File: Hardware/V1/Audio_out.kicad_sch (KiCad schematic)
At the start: 30 parts, among them J0 0, J1 SJ2-3514A-SMT-TR, Q1 BC817-25-QVL

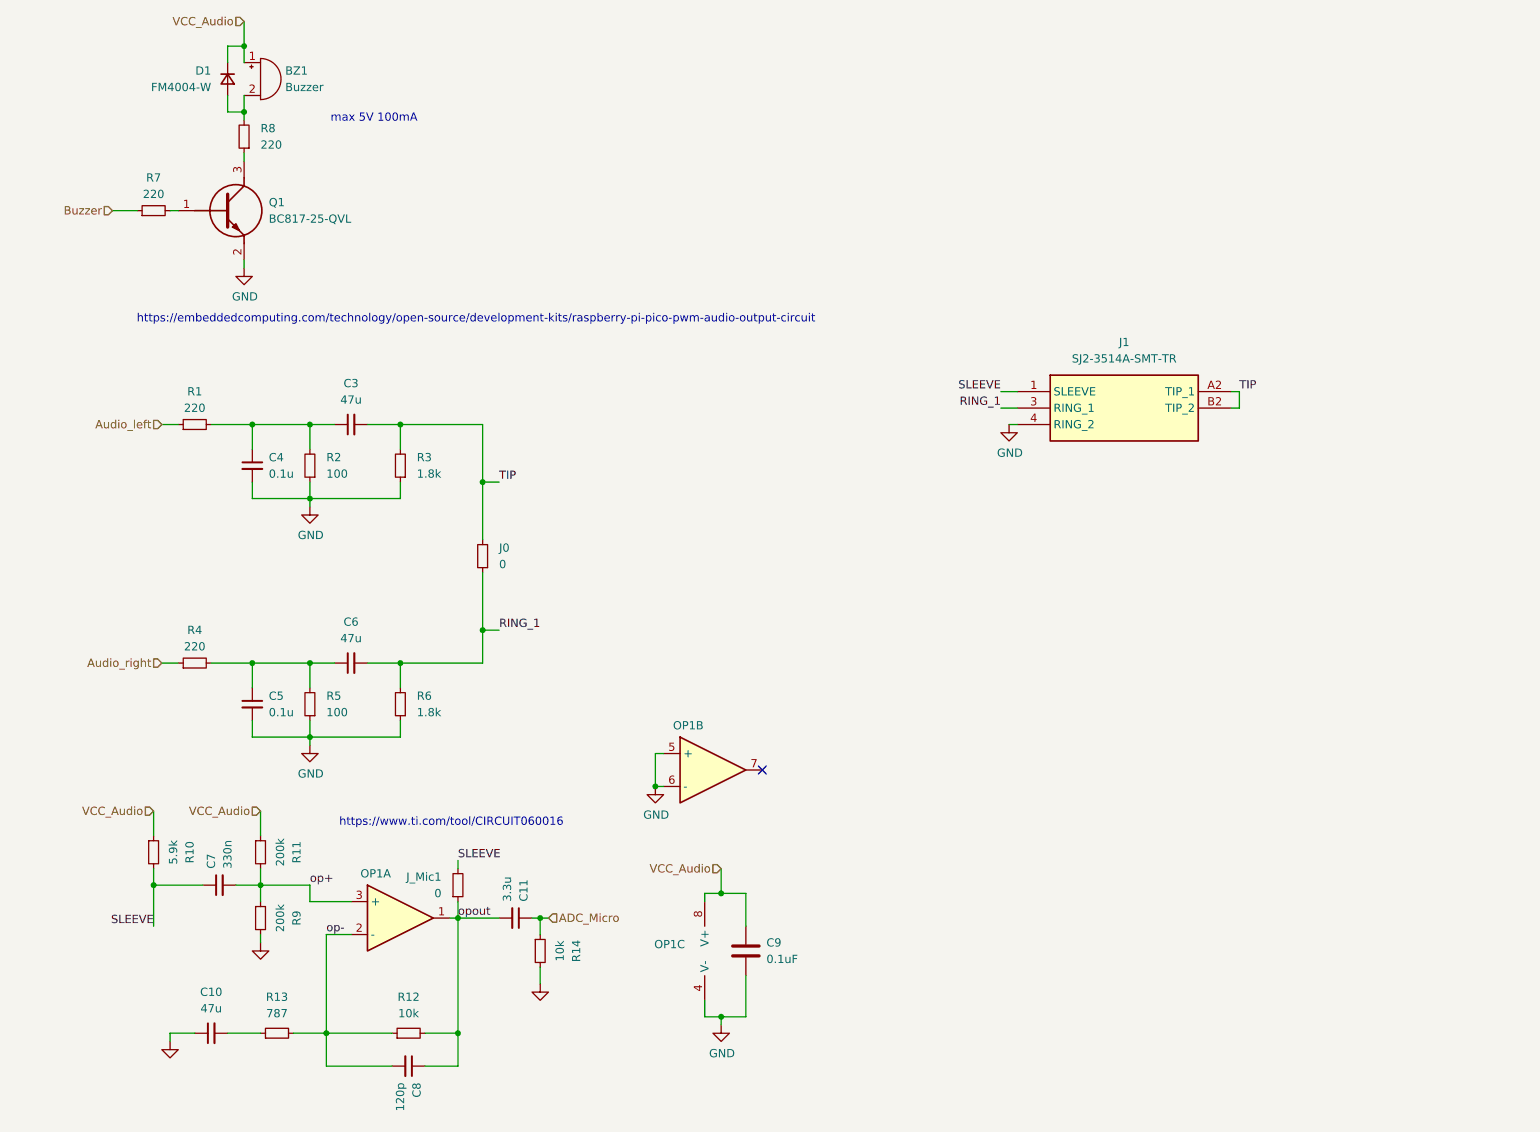
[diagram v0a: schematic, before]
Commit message: asd
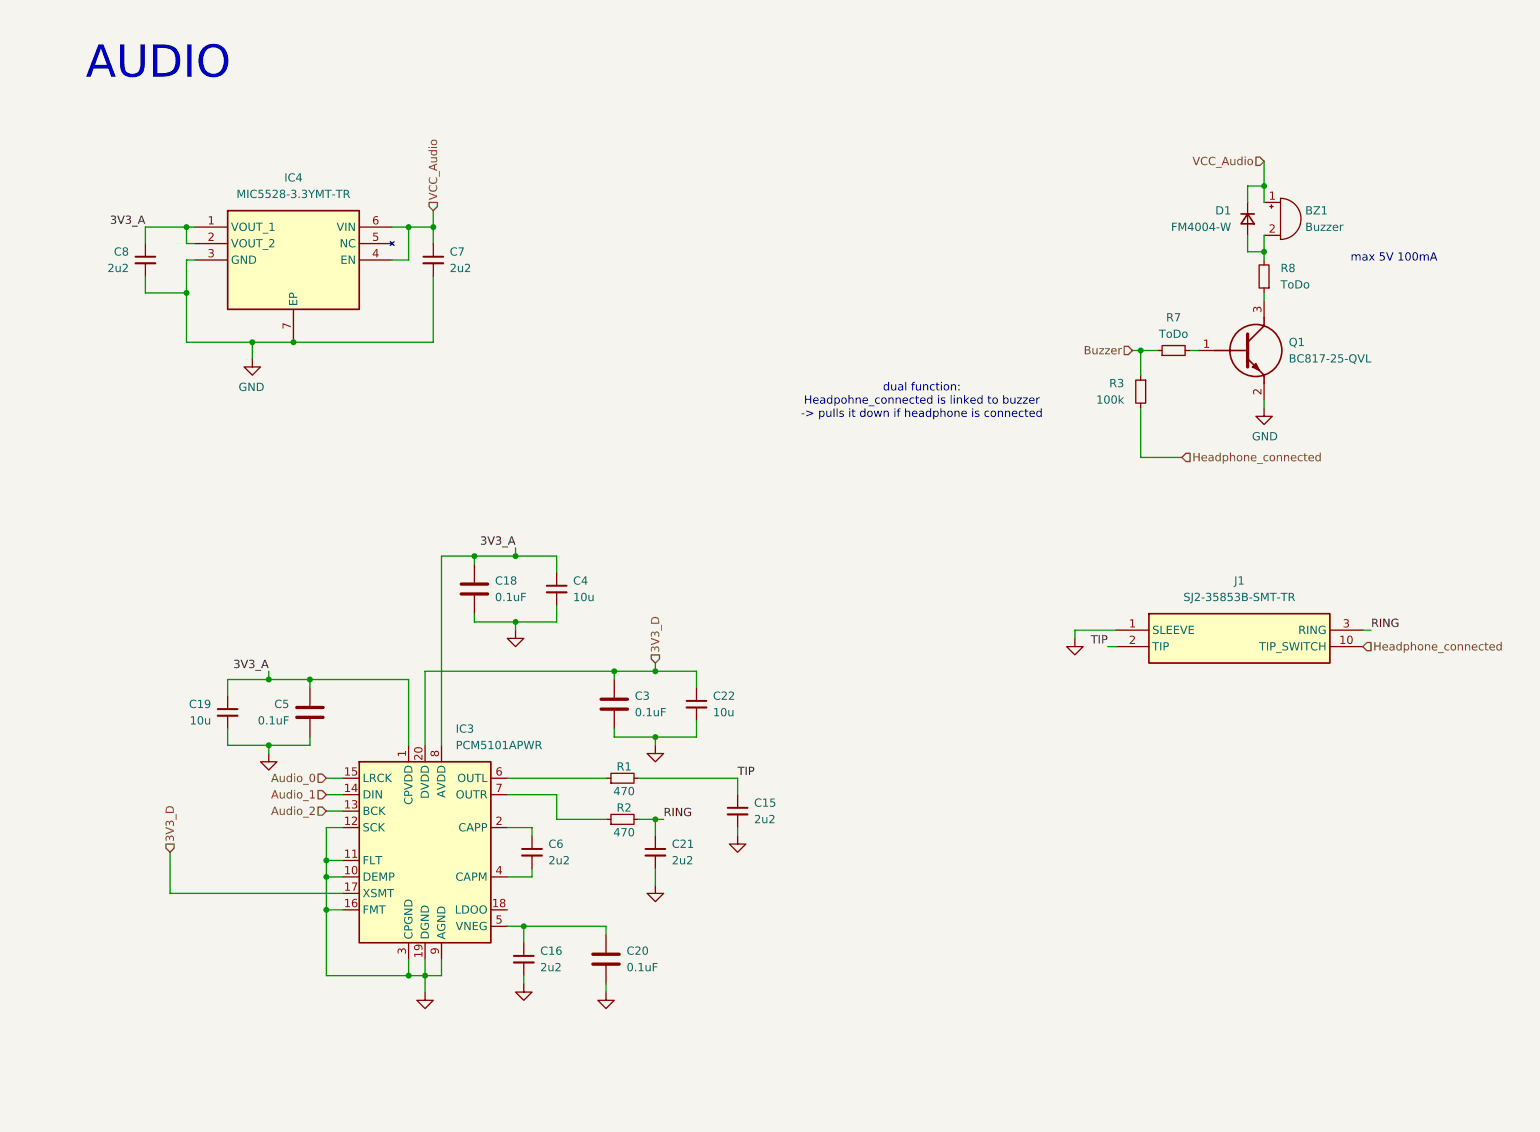
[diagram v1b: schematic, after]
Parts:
- removed C10, C3: 47u, Capacitor_SMD:C_1206_3216Metric_Pad1.33x1.80mm_HandSolder, symbol Device:C_Small
- removed C11: 3.3u, Capacitor_SMD:C_0805_2012Metric_Pad1.18x1.45mm_HandSolder, symbol Device:C_Small
- removed C5: 0.1u, Capacitor_SMD:C_0402_1005Metric, symbol Device:C_Small
- removed C9: 0.1uF, Capacitor_SMD:C_0402_1005Metric_Pad0.74x0.62mm_HandSolder, symbol SymbolsBalloonv4:C
- removed J0, J_Mic1: 0, Resistor_SMD:R_0603_1608Metric, symbol Device:R_Small
- removed J1: SJ2-3514A-SMT-TR, SamacSys_Parts:SJ23514ASMTTR, symbol SamacSys_Parts:SJ2-3514A-SMT-TR
- removed OP1: TLV9002QDRQ1, SamacSys_Parts:SOIC127P600X175-8N, symbol SymbolsBalloonv4:Opamp_Dual
- removed R1, R4: 220, Resistor_SMD:R_0603_1608Metric, symbol Device:R_Small
- removed R10: 5.9k, Resistor_SMD:R_0603_1608Metric_Pad0.98x0.95mm_HandSolder, symbol SymbolsBalloonv4:R_Small
- removed R11, R9: 200k, Resistor_SMD:R_0603_1608Metric_Pad0.98x0.95mm_HandSolder, symbol SymbolsBalloonv4:R_Small
- removed R12, R14: 10k, Resistor_SMD:R_0603_1608Metric_Pad0.98x0.95mm_HandSolder, symbol SymbolsBalloonv4:R_Small
- removed R13: 787, Resistor_SMD:R_0603_1608Metric_Pad0.98x0.95mm_HandSolder, symbol SymbolsBalloonv4:R_Small
- removed R2, R5: 100, Resistor_SMD:R_0603_1608Metric, symbol Device:R_Small
- removed R6: 1.8k, Resistor_SMD:R_0603_1608Metric, symbol Device:R_Small
- added C15, C16, C21: 2u2, SamacSys_Parts:CAPC1608X90N, symbol Device:C_Small
- added C18, C20, C3, C5: 0.1uF, Capacitor_SMD:C_0402_1005Metric_Pad0.74x0.62mm_HandSolder, symbol SymbolsBalloonv4:C
- added C19, C22: 10u, SamacSys_Parts:CAPC1608X50N, symbol Device:C_Small
- added IC3: PCM5101APWR, Package_SO:TSSOP-20_4.4x6.5mm_P0.65mm, symbol Audio:PCM5101A
- added IC4: MIC5528-3.3YMT-TR, SamacSys_Parts:SON40P120X120X60-7N-D, symbol SamacSys_Parts:MIC5528-3.3YMT-TR
- added J1: SJ2-35853B-SMT-TR, SamacSys_Parts:SJ235853BSMTTR, symbol SamacSys_Parts:SJ2-35853B-SMT-TR
- added R1, R2: 470, Resistor_SMD:R_0603_1608Metric_Pad0.98x0.95mm_HandSolder, symbol SymbolsBalloonv4:R_Small
- C4: value 0.1u -> 10u; footprint Capacitor_SMD:C_0402_1005Metric -> SamacSys_Parts:CAPC1608X50N; Height (none) -> 0.5; Manufacturer_Name (none) -> TAIYO YUDEN; Manufacturer_Part_Number (none) -> JMK107ABJ106MA-T; Mouser Part Number (none) -> 963-JMK107ABJ106MA-T; Mouser Price/Stock (none) -> https://www.mouser.co.uk/ProductDetail/Taiyo-Yuden/JMK107AB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
- C6: value 47u -> 2u2; footprint Capacitor_SMD:C_1206_3216Metric_Pad1.33x1.80mm_HandSolder -> SamacSys_Parts:CAPC1608X90N; Height (none) -> 0.9; Manufacturer_Name (none) -> TAIYO YUDEN; Manufacturer_Part_Number (none) -> LMK107BJ225KA-T; Mouser Part Number (none) -> 963-LMK107BJ225KA-T; Mouser Price/Stock (none) -> https://www.mouser.co.uk/ProductDetail/TAIYO-YUDEN/LMK107BJ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
- C7: value 330n -> 2u2; footprint Capacitor_SMD:C_0805_2012Metric_Pad1.18x1.45mm_HandSolder -> SamacSys_Parts:CAPC1608X90N; Height (none) -> 0.9; Manufacturer_Name (none) -> TAIYO YUDEN; Manufacturer_Part_Number (none) -> LMK107BJ225KA-T; Mouser Part Number (none) -> 963-LMK107BJ225KA-T; Mouser Price/Stock (none) -> https://www.mouser.co.uk/ProductDetail/TAIYO-YUDEN/LMK107BJ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
- C8: value 120p -> 2u2; footprint Capacitor_SMD:C_0805_2012Metric_Pad1.18x1.45mm_HandSolder -> SamacSys_Parts:CAPC1608X90N; Height (none) -> 0.9; Manufacturer_Name (none) -> TAIYO YUDEN; Manufacturer_Part_Number (none) -> LMK107BJ225KA-T; Mouser Part Number (none) -> 963-LMK107BJ225KA-T; Mouser Price/Stock (none) -> https://www.mouser.co.uk/ProductDetail/TAIYO-YUDEN/LMK107BJ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
- R3: value 1.8k -> 100k
- R7, R8: value 220 -> ToDo
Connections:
- net SLEEVE is gone; now on net VCC_Audio: C7.1
- net op+ is gone; now on net GND: C7.2
- net op- is gone; now on net GND: C8.2
- net opout is gone; now on net 3V3_A: C8.1
- net Buzzer: now also R3.1
- net GND: now also C15.2, C16.2, C18.1, C19.2, C20.1, C21.2, C22.2, C3.1, C5.1, IC3.10 (DEMP), IC3.11 (FLT), IC3.12 (SCK), IC3.16 (FMT), IC3.19 (DGND), IC3.3 (CPGND), IC3.9 (AGND), IC4.3 (GND), IC4.7 (EP), J1.1 (SLEEVE); no longer R3.1
- net TIP: now also C15.1, J1.2 (TIP), R1.2; no longer R3.2
- net VCC_Audio: now also IC4.4 (EN), IC4.6 (VIN)
- net 3V3_A: now reaches C4.1
- net 3V3_A: now also C18.2, C19.1, C5.2, IC3.1 (CPVDD), IC3.8 (AVDD), IC4.1 (VOUT_1), IC4.2 (VOUT_2)
- net at C6.1: now also IC3.2 (CAPP)
- net RING_1: no longer names the net of C6.2
- net RING_1: now also IC3.4 (CAPM)
- new net: C16.1, C20.2, IC3.5 (VNEG)
- new net: IC3.6 (OUTL), R1.1
- new net: IC3.7 (OUTR), R2.1
- new net 3V3_D: C22.1, C3.2, IC3.17 (XSMT), IC3.20 (DVDD)
- new net Audio_0: IC3.15 (LRCK)
- new net Audio_1: IC3.14 (DIN)
- new net Audio_2: IC3.13 (BCK)
- new net Headphone_connected: J1.10 (TIP_SWITCH), R3.2
- new net RING: C21.1, J1.3 (RING), R2.2
- no-connect marks 1 -> 0
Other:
- note added: "AUDIO"
- note added: "dual function: Headpohne_connected is linked to buzzer -> pulls it down if headphone is connected"
- note removed: "https://embeddedcomputing.com/technology/open-source/development-kits/raspberry-pi-pico-pwm-audio-output-circuit"
- note removed: "https://www.ti.com/tool/CIRCUIT060016"
- moved on the sheet: BZ1, D1, Q1, R7, R8
